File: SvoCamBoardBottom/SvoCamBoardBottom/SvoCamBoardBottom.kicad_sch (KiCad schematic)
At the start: 15 parts, among them J1 Conn_01x02_Pin, J2 43650-0528, Q1 BC817, Q2 BC817, Q3 BC817, U1 ESP32-CAM, U3 FT232RL

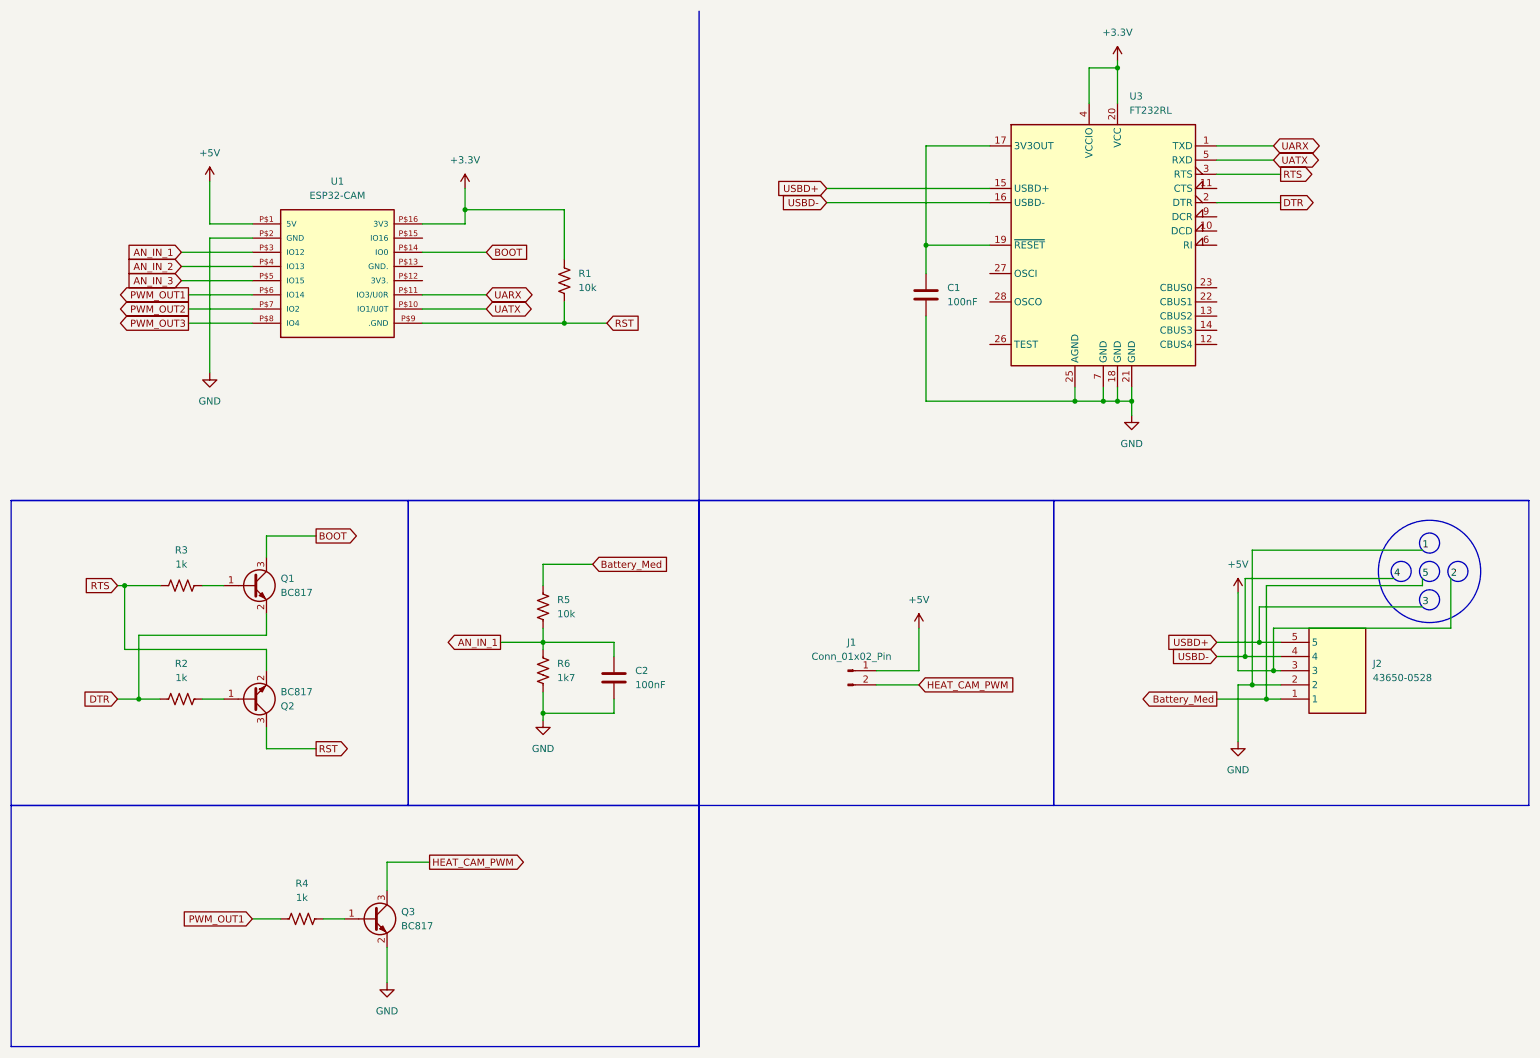
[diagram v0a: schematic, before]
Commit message: svocanboard
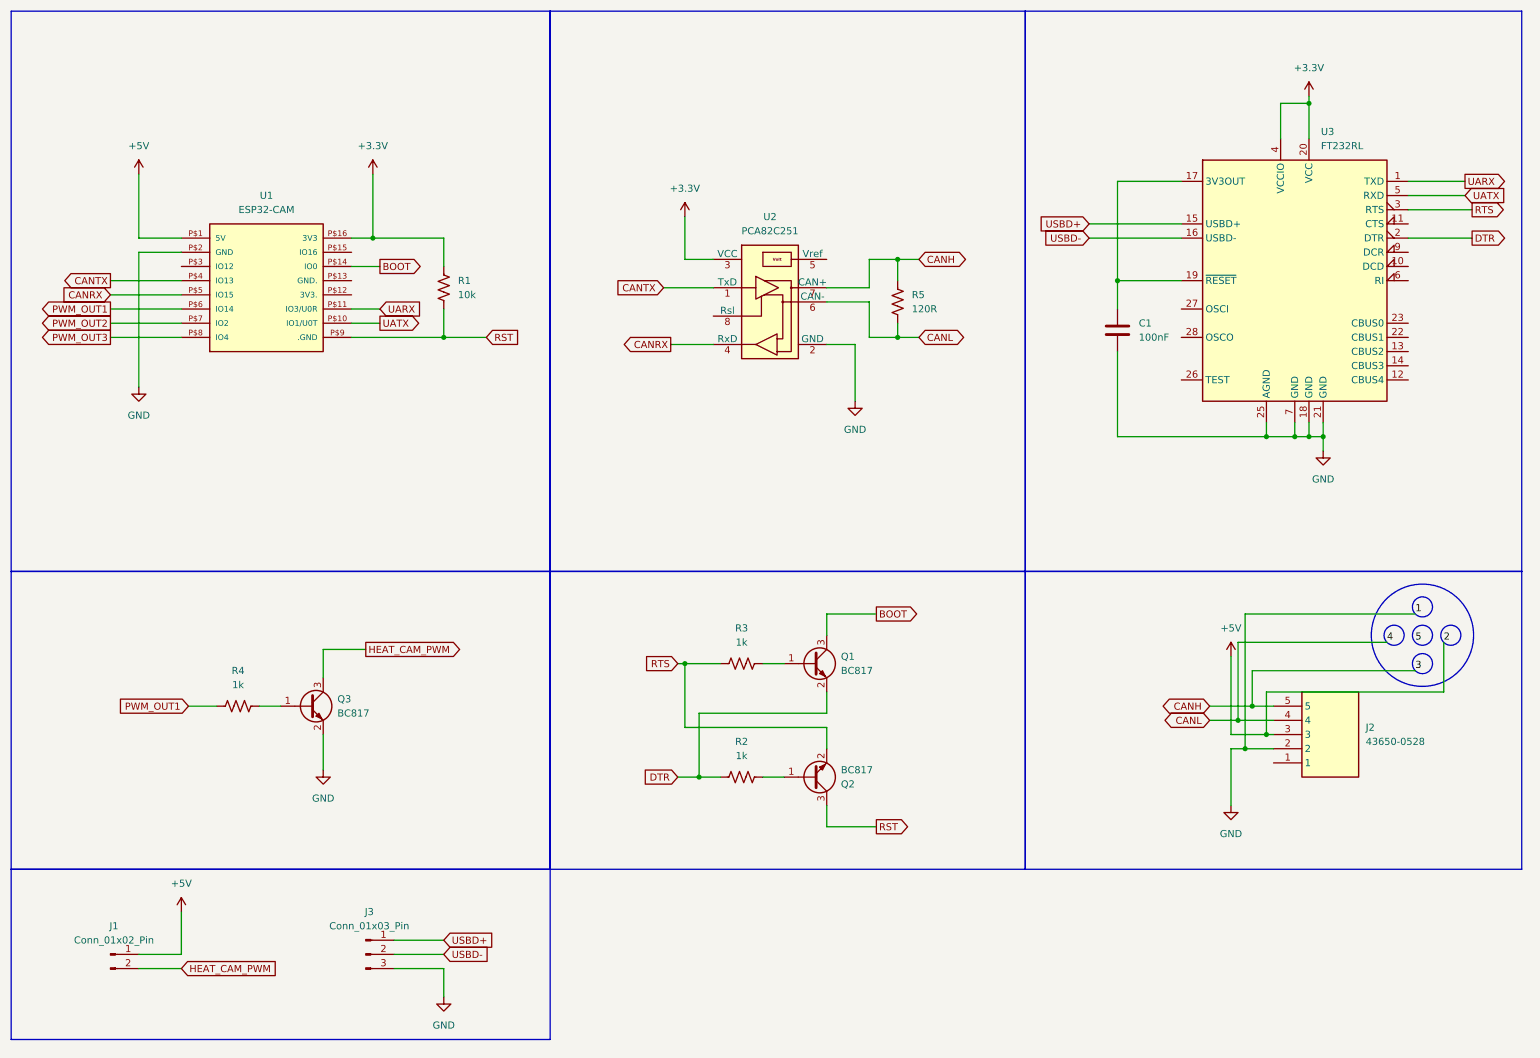
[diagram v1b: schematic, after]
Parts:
- removed C2: 100nF, Capacitor_SMD:C_0805_2012Metric, symbol Device:C
- removed R6: 1k7, Resistor_SMD:R_0805_2012Metric, symbol Device:R_US
- added J3: Conn_01x03_Pin, Connector_PinSocket_2.54mm:PinSocket_1x03_P2.54mm_Vertical, symbol Connector:Conn_01x03_Pin
- added U2: PCA82C251, Package_SO:SO-8_3.9x4.9mm_P1.27mm, symbol Interface_CAN_LIN:PCA82C251
- C1: footprint Capacitor_SMD:C_01005_0402Metric -> Capacitor_SMD:C_0805_2012Metric
- R5: value 10k -> 120R
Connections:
- net +3.3V: now also U2.3 (VCC)
- net GND: now also J3.3 (Pin_3), U2.2 (GND)
- net USBD+: now also J3.1 (Pin_1); no longer J2.5
- net USBD-: now also J3.2 (Pin_2); no longer J2.4
- net AN_IN_1: no longer names the net of U1.P$3 (IO12)
- net AN_IN_1: no longer R5.2
- net AN_IN_2 renamed CANTX
- net CANTX: now also U2.1 (TxD)
- net AN_IN_3 renamed CANRX
- net CANRX: now also U2.4 (RxD)
- net Battery_Med: no longer names the net of J2.1
- net Battery_Med: no longer R5.1
- new net CANH: J2.5, R5.1, U2.7 (CAN+)
- new net CANL: J2.4, R5.2, U2.6 (CAN-)
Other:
- moved on the sheet: C1, J1, J2, Q1, Q2, Q3, R1, R2, R3, R4, U1, U3

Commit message: svocamboard
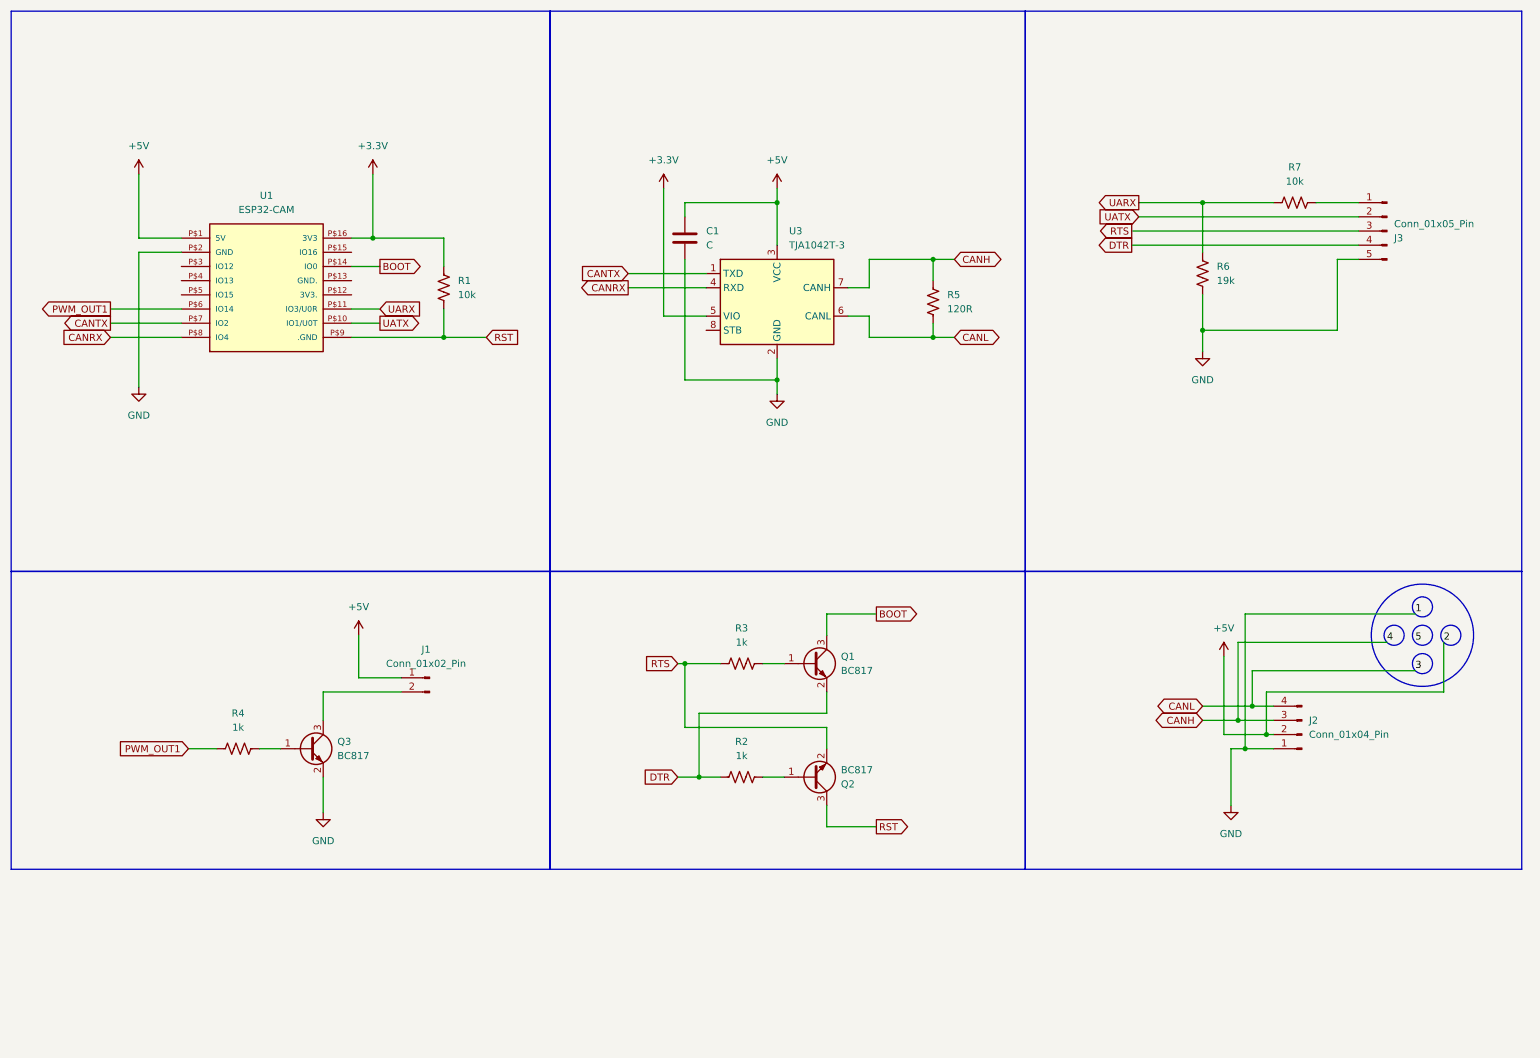
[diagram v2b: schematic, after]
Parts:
- removed J2: 43650-0528, Esp32_Conn_Cam:43650-05YY_272829, symbol Conn_Esp32_Cam:43650-0528
- removed J3: Conn_01x03_Pin, Connector_PinSocket_2.54mm:PinSocket_1x03_P2.54mm_Vertical, symbol Connector:Conn_01x03_Pin
- removed U2: PCA82C251, Package_SO:SO-8_3.9x4.9mm_P1.27mm, symbol Interface_CAN_LIN:PCA82C251
- removed U3: FT232RL, Package_SO:SSOP-28_5.3x10.2mm_P0.65mm, symbol Interface_USB:FT232RL
- added J2: Conn_01x04_Pin, Connector_PinHeader_2.54mm:PinHeader_1x04_P2.54mm_Vertical, symbol Connector:Conn_01x04_Pin
- added J3: Conn_01x05_Pin, Connector_PinHeader_2.54mm:PinHeader_1x05_P2.54mm_Vertical, symbol Connector:Conn_01x05_Pin
- added R6: 19k, Resistor_SMD:R_0805_2012Metric, symbol Device:R_US
- added R7: 10k, Resistor_SMD:R_0805_2012Metric, symbol Device:R_US
- added U3: TJA1042T-3, Package_SO:SOIC-8_3.9x4.9mm_P1.27mm, symbol Interface_CAN_LIN:TJA1042T-3
- C1: value 100nF -> C; footprint Capacitor_SMD:C_0805_2012Metric -> Capacitor_SMD:C_1206_3216Metric
- U1: footprint Esp32:ESP32-CAM -> esp32:ESP32-CAM
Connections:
- net PWM_OUT2 is gone; now on net CANTX: U1.P$7 (IO2)
- net PWM_OUT3 is gone; now on net CANRX: U1.P$8 (IO4)
- net +3.3V: now also U3.5 (VIO)
- net +5V: now also C1.1, J2.2 (Pin_2), U3.3 (VCC)
- net CANH: now also J2.3 (Pin_3), U3.7 (CANH)
- net CANL: now also J2.4 (Pin_4), U3.6 (CANL)
- net CANRX: now also U3.4 (RXD); no longer U1.P$5 (IO15)
- net CANTX: now also U3.1 (TXD); no longer U1.P$4 (IO13)
- net DTR: now also J3.4 (Pin_4)
- net GND: now also J2.1 (Pin_1), J3.5 (Pin_5), R6.2, U3.2 (GND)
- net RTS: now also J3.3 (Pin_3)
- net UARX: now also R6.1, R7.1
- net UATX: now also J3.2 (Pin_2)
- net HEAT_CAM_PWM: no longer names the net of J1.2 (Pin_2), Q3.3 (C)
- new net: J3.1 (Pin_1), R7.2
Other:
- moved on the sheet: J1, Q3, R4, R5
